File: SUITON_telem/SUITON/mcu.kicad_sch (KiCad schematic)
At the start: 22 parts, among them U1 STM32H523ZCT6

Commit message: Flash mode
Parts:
- added C21, C22: 12pF, Capacitor_SMD:C_0603_1608Metric, symbol Device:C
- added C23, C24: 100nF, Capacitor_SMD:C_0603_1608Metric, symbol Device:C
- added J1: USB_C_Receptacle_USB2.0_14P, symbol Connector:USB_C_Receptacle_USB2.0_14P
- added R2: 47 Ω, symbol Device:R
- added R3, R4: 5.1kΩ, symbol Device:R
- added S1, S2: B3U-1000P, B3U-1000P:SW_B3U-1000P, symbol B3U-1000P:B3U-1000P
- added X1: ABM3B-8.000MHZ-10-1UT, XTAL4P_ABM3B_ABR, symbol 2026-09-29_10-16-59:ABM3B-8.000MHZ-10-1UT
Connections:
- net +3V3: now also S2.1
- net GND: now also C21.2, C22.2, C23.2, C24.2, J1.A1 (GND), J1.A12 (GND), J1.B1 (GND), J1.B12 (GND), J1.S1 (SHIELD), R2.2, R3.2, R4.2, S1.1, X1.2, X1.4
- net BOOT: now reaches U1.138 (BOOT0)
- net BOOT: now also C24.1, R2.1, S2.2
- net OSC_IN: now reaches U1.23 (PH0-OSC_IN)
- net OSC_IN: now also C22.1, X1.1
- net OSC_OUT: now reaches U1.24 (PH1-OSC_OUT)
- net OSC_OUT: now also C21.1, X1.3
- net NRST: now reaches U1.25 (NRST)
- net NRST: now also C23.1, S1.2
- net USB_DM: now reaches U1.103 (PA11)
- net USB_DM: now also J1.A7 (D-), J1.B7 (D-)
- net USB_DP: now reaches U1.104 (PA12)
- net USB_DP: now also J1.A6 (D+), J1.B6 (D+)
- net SWDIO: now reaches U1.105 (PA13)
- net SWCLK: now reaches U1.109 (PA14)
- net SWO: now reaches U1.133 (PB3)
- new net: J1.B5 (CC2), R4.1
- new net: J1.A5 (CC1), R3.1
- new net +5V_USB: J1.A4 (VBUS), J1.A9 (VBUS), J1.B4 (VBUS), J1.B9 (VBUS)
- no-connect marks 0 -> 2
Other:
- moved on the sheet: C1, C10, C11, C12, C13, C14, C15, C16, C17, C18, C19, C2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

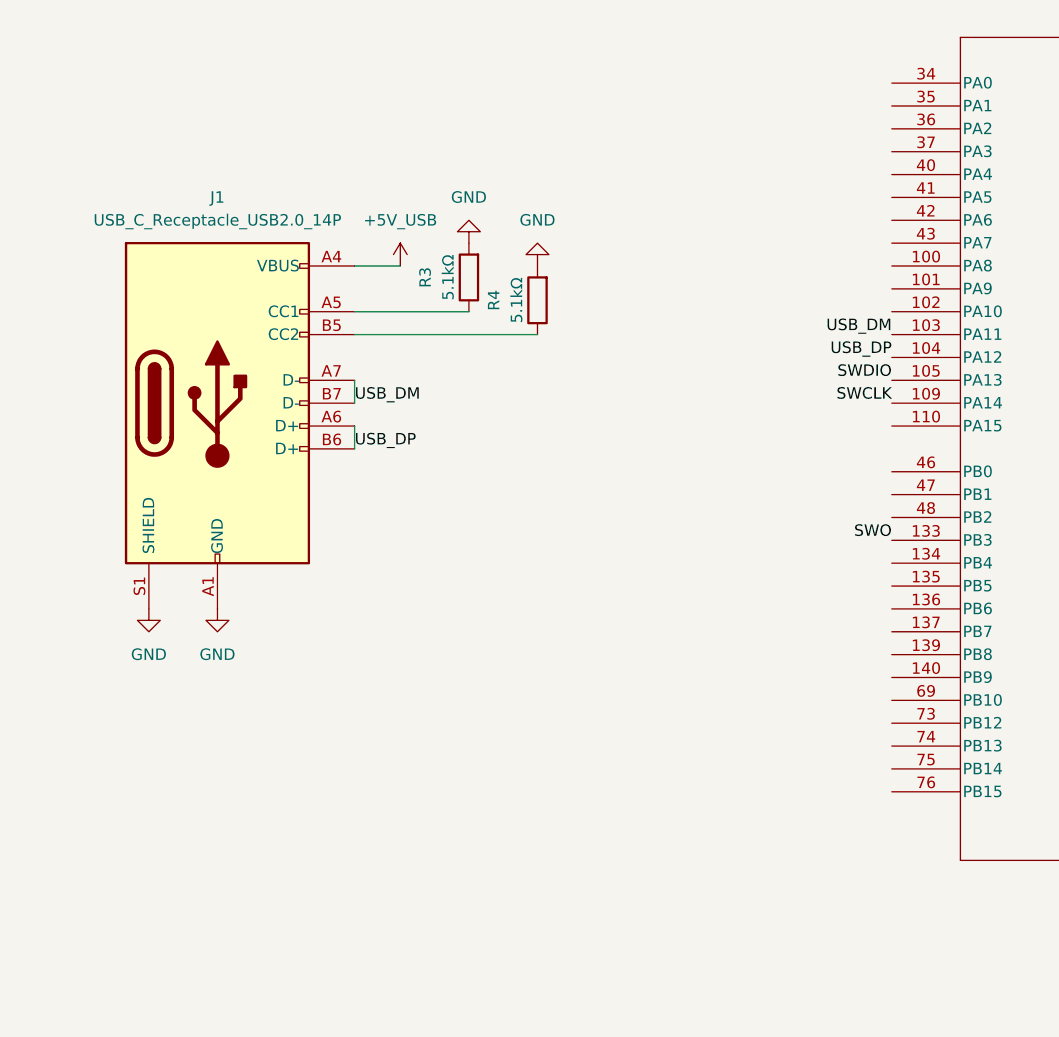
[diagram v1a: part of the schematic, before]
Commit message: Sensor
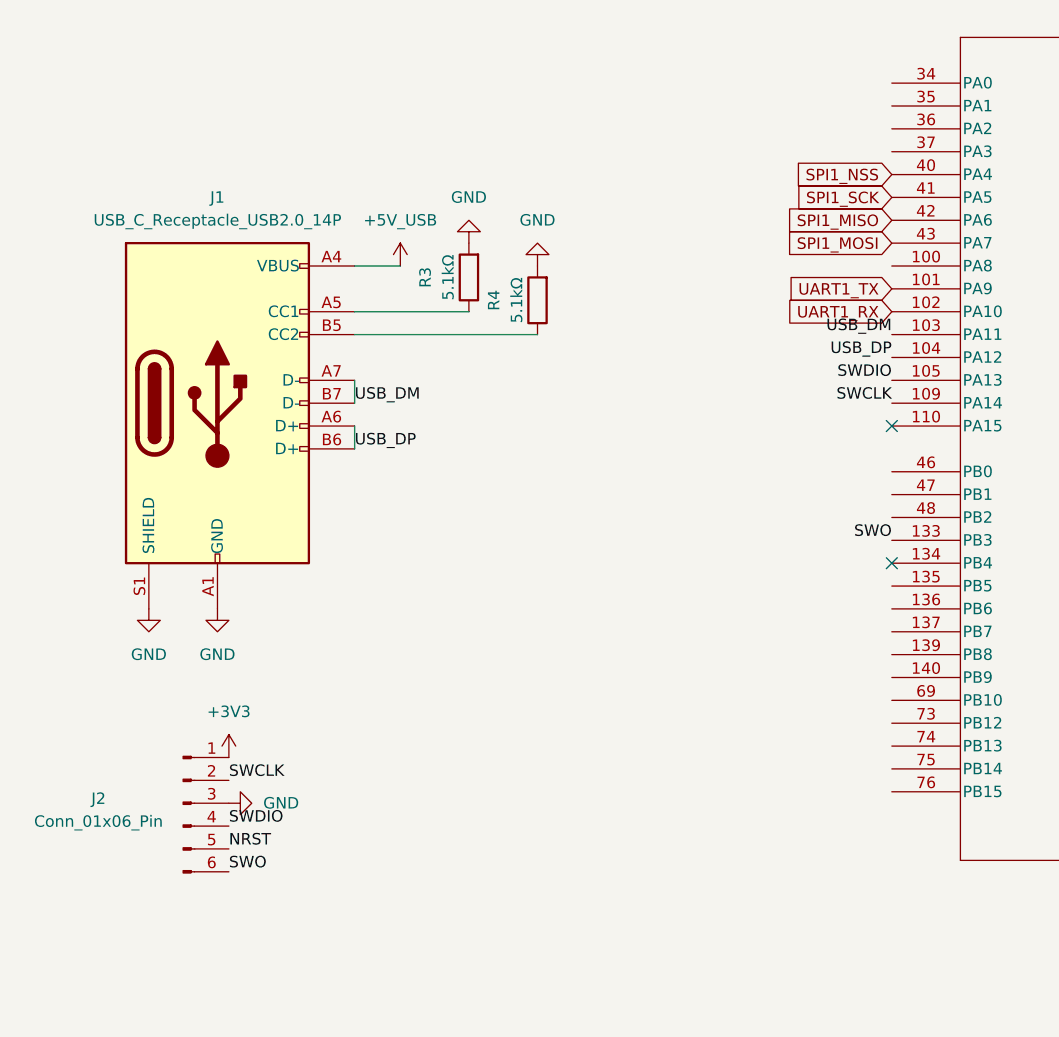
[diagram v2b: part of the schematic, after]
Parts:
- added J2: Conn_01x06_Pin, symbol Connector:Conn_01x06_Pin
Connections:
- net +3V3: now also J2.1 (Pin_1)
- net GND: now also J2.3 (Pin_3)
- net NRST: now also J2.5 (Pin_5)
- net SWCLK: now also J2.2 (Pin_2)
- net SWDIO: now also J2.4 (Pin_4)
- net SWO: now also J2.6 (Pin_6)
- net UART1_TX: now reaches U1.101 (PA9)
- net UART1_RX: now reaches U1.102 (PA10)
- net SPI1_NSS: now reaches U1.40 (PA4)
- net SPI1_SCK: now reaches U1.41 (PA5)
- net SPI1_MISO: now reaches U1.42 (PA6)
- net SPI1_MOSI: now reaches U1.43 (PA7)
- no-connect marks 2 -> 4

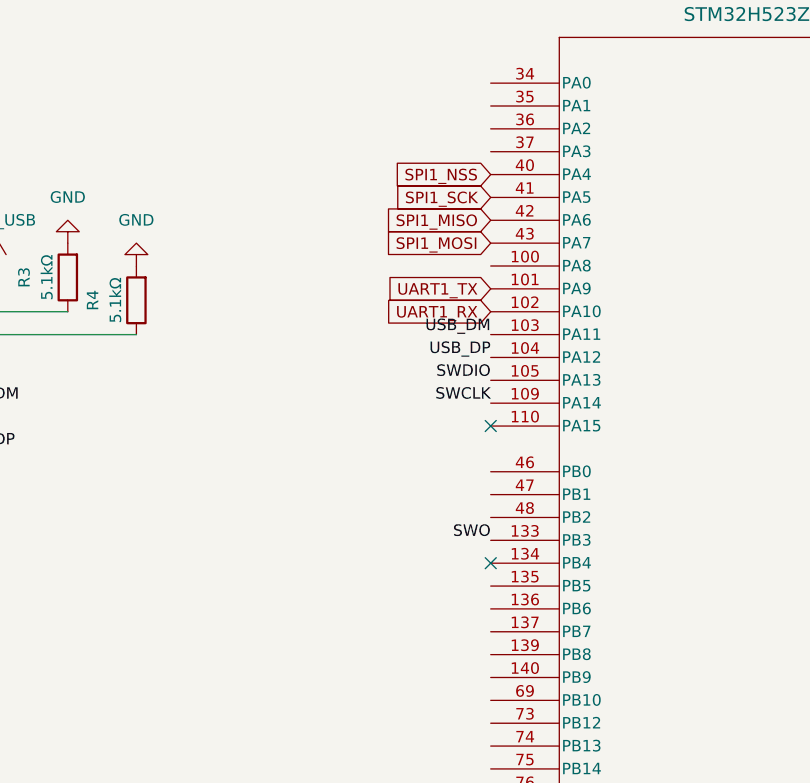
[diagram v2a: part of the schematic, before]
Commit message: power management
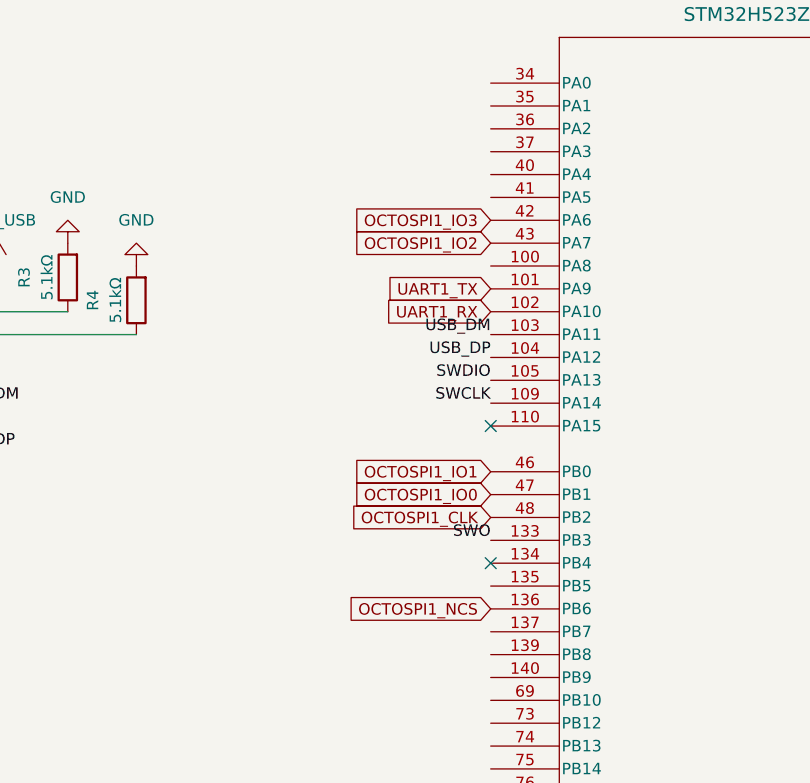
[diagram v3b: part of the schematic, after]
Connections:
- net OCTOSPI1_NCS: now reaches U1.136 (PB6)
- net OCTOSPI1_IO1: now reaches U1.46 (PB0)
- net OCTOSPI1_IO0: now reaches U1.47 (PB1)
- net OCTOSPI1_CLK: now reaches U1.48 (PB2)
- net SPI1_MISO renamed OCTOSPI1_IO3
- net SPI1_MOSI renamed OCTOSPI1_IO2
- net SPI1_NSS: no longer names the net of U1.40 (PA4)
- net SPI1_SCK: no longer names the net of U1.41 (PA5)
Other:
- company: (none) -> S.T.A.R.
- title: (none) -> SUITON PRO
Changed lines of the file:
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@@
 	(generator_version "8.0")
 	(paper "A3")
+	(title_block
+		(title "SUITON PRO")
+		(date "2026-10-01")
+		(company "S.T.A.R.")
+		(comment 1 "Axel BOULAROT")
+		(comment 2 "Versatile Flight Controller for rocket and more")
+	)
 	(junction
 		(at 304.8 168.91)
@@
 		)
 	)
-	(global_label "SPI1_MOSI"
+	(global_label "OCTOSPI1_IO1"
 		(shape input)
-		(at 111.76 64.77 180)
+		(at 111.76 90.17 180)
 		(fields_autoplaced yes)
 		(effects
@@
 		)
 		(property "Intersheetrefs" "${INTERSHEET_REFS}"
-			(at 98.9172 64.77 0)
+			(at 95.47 90.17 0)
 			(effects
 				(font
@@
 		)
 	)
-	(global_label "SPI1_SCK"
+	(global_label "OCTOSPI1_CLK"
 		(shape input)
-		(at 111.76 59.69 180)
+		(at 111.76 95.25 180)
 		(fields_autoplaced yes)
 		(effects
@@
 		)
 		(property "Intersheetrefs" "${INTERSHEET_REFS}"
-			(at 99.7639 59.69 0)
+			(at 95.0467 95.25 0)
 			(effects
 				(font
@@
 		)
 	)
-	(global_label "SPI1_MISO"
+	(global_label "OCTOSPI1_IO3"
 		(shape input)
 		(at 111.76 62.23 180)
@@
 		)
 		(property "Intersheetrefs" "${INTERSHEET_REFS}"
-			(at 98.9172 62.23 0)
+			(at 95.47 62.23 0)
 			(effects
 				(font
@@
 		)
 	)
-	(global_label "SPI1_NSS"
+	(global_label "OCTOSPI1_IO0"
 		(shape input)
-		(at 111.76 57.15 180)
+		(at 111.76 92.71 180)
 		(fields_autoplaced yes)
 		(effects
@@
 		)
 		(property "Intersheetrefs" "${INTERSHEET_REFS}"
-			(at 99.7639 57.15 0)
+			(at 95.47 92.71 0)
 			(effects
 				(font
+					(size 1.27 1.27)
+				)
+				(justify right)
+				(hide yes)
+			)
+		)
+	)
+	(global_label "OCTOSPI1_IO2"
+		(shape input)
+		(at 111.76 64.77 180)
+		(fields_autoplaced yes)
+		(effects
+			(font
+				(size 1.27 1.27)
+			)
+			(justify right)
+		)
+		(property "Intersheetrefs" "${INTERSHEET_REFS}"
+			(at 95.47 64.77 0)
+			(effects
+				(font
+					(size 1.27 1.27)
+				)
+				(justify right)
+				(hide yes)
+			)
+		)
+	)
+	(global_label "OCTOSPI1_NCS"
+		(shape input)
+		(at 111.76 105.41 180)
+		(fields_autoplaced yes)
+		(effects
+			(font
+				(size 1.27 1.27)
+			)
+			(justify right)
+		)
+		(property "Intersheetrefs" "${INTERSHEET_REFS}"
+			(at 94.8048 105.41 0)
+			(effects
+				(font
